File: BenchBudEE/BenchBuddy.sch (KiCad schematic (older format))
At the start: 0 parts

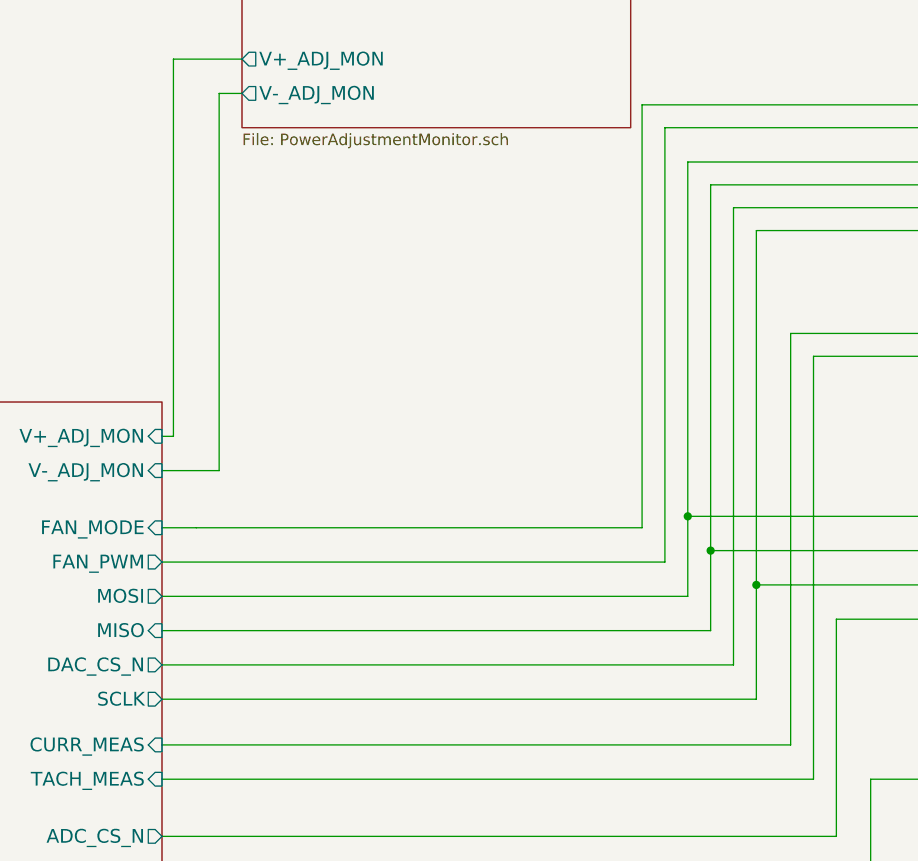
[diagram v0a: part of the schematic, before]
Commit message: playing with the layout
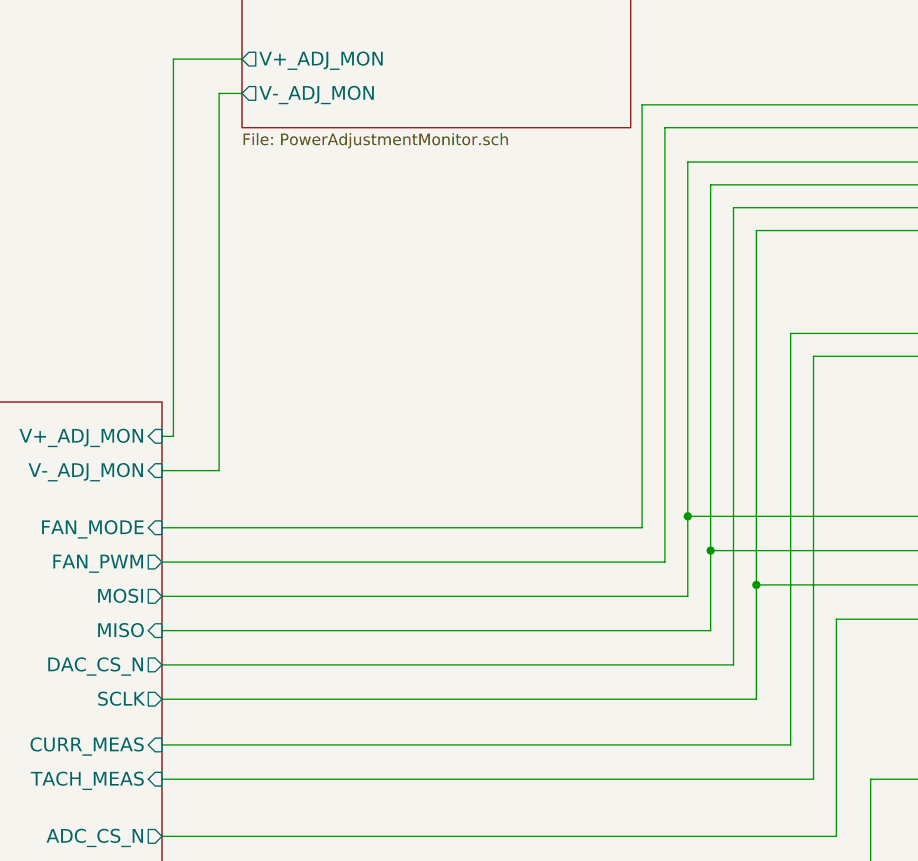
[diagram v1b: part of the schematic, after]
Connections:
- wire segments 58 -> 53
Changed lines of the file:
@@
-EESchema Schematic File Version 2  date 10/10/2013 12:18:22 AM
+EESchema Schematic File Version 2
 LIBS:power
 LIBS:device
@@
 Sheet 1 9
 Title "noname.sch"
-Date "10 oct 2013"
+Date "3 mar 2014"
 Rev ""
 Comp ""
@@
 	7750 2350 6700 2350
 Wire Wire Line
-	6700 2350 6700 3900
-Wire Wire Line
-	6700 3900 6700 4250
+	6700 2350 6700 4250
 Wire Wire Line
 	6700 4250 4400 4250
@@
 	7750 2450 6800 2450
 Wire Wire Line
-	6800 2450 6800 4050
-Wire Wire Line
-	6800 4050 6800 4400
+	6800 2450 6800 4400
 Wire Wire Line
 	6800 4400 4400 4400
@@
 	6900 2550 6900 4550
 Wire Wire Line
-	7000 2650 7000 4200
-Wire Wire Line
-	7000 4200 7000 4700
+	7000 2650 7000 4700
 Wire Wire Line
 	7000 4700 4400 4700
@@
 	6500 3950 6500 2100
 Wire Wire Line
-	4550 3950 6500 3950
-Wire Wire Line
-	4550 3950 4550 3950
-Wire Wire Line
-	4550 3950 4400 3950
+	4400 3950 6500 3950
 $EndSCHEMATC
